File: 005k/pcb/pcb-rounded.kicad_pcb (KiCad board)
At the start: 2 copper layers, 293.2 x 106 mm, 107 parts, among them J1 Screw_Terminal_01x04, U1 ProMicro

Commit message: dim. 10 déc. 2023 13:12:07 CET
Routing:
- net C6: track 234.3 -> 222.5 mm
- net C5: track 287.5 -> 298.1 mm
- net C1: track 426.7 -> 416.5 mm
- net C3: track 419.0 -> 424.1 mm
- net L8: track 210.1 -> 214.1 mm
- net L5: track 143.8 -> 145.8 mm
- net C4: track 334.0 -> 336.0 mm
- net L7: track 153.2 -> 155.0 mm
- net L6: track 138.0 -> 139.7 mm
- net C2: track 438.7 -> 437.7 mm, vias 1 -> 0
- net L1: track 159.0 -> 158.3 mm

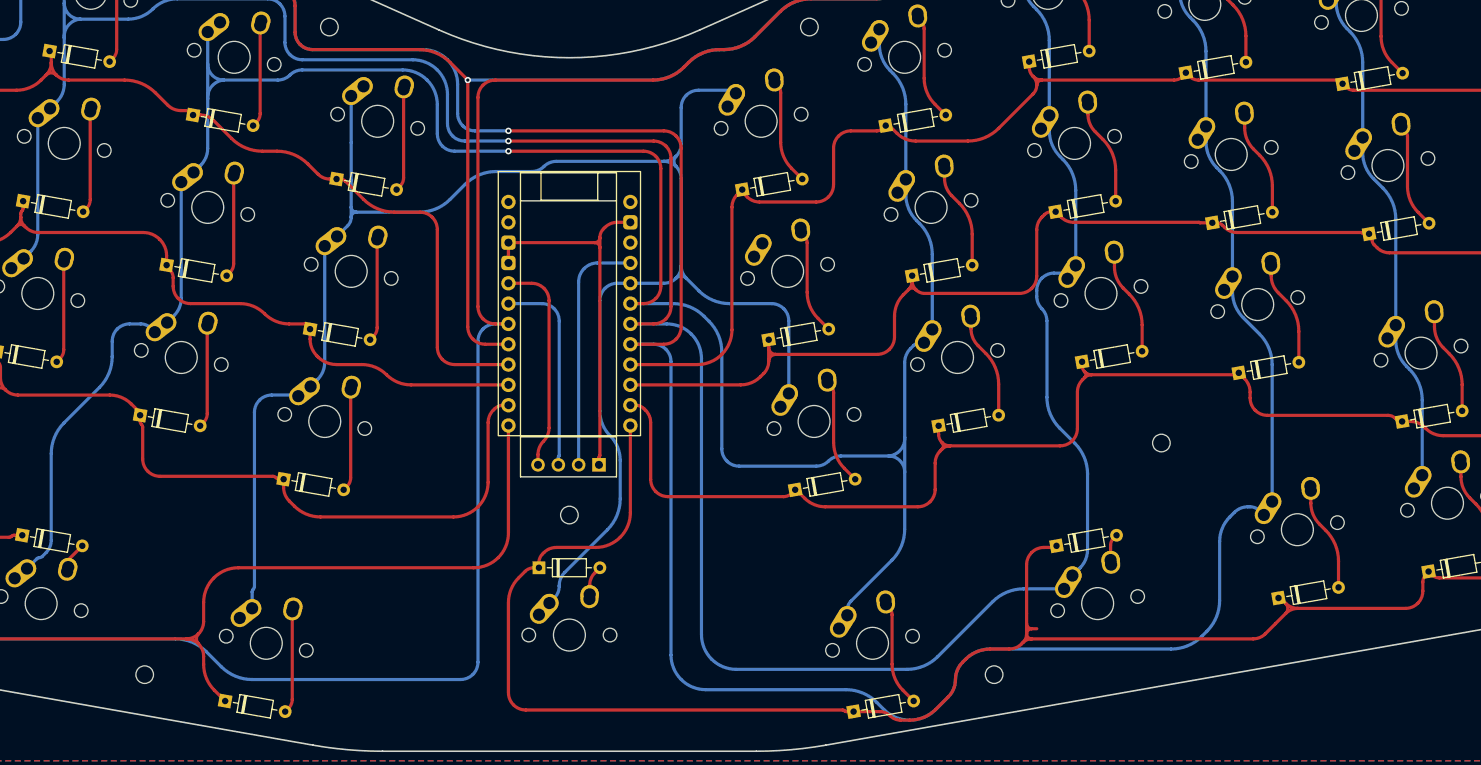
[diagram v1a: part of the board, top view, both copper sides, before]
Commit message: dim. 10 déc. 2023 20:23:19 CET
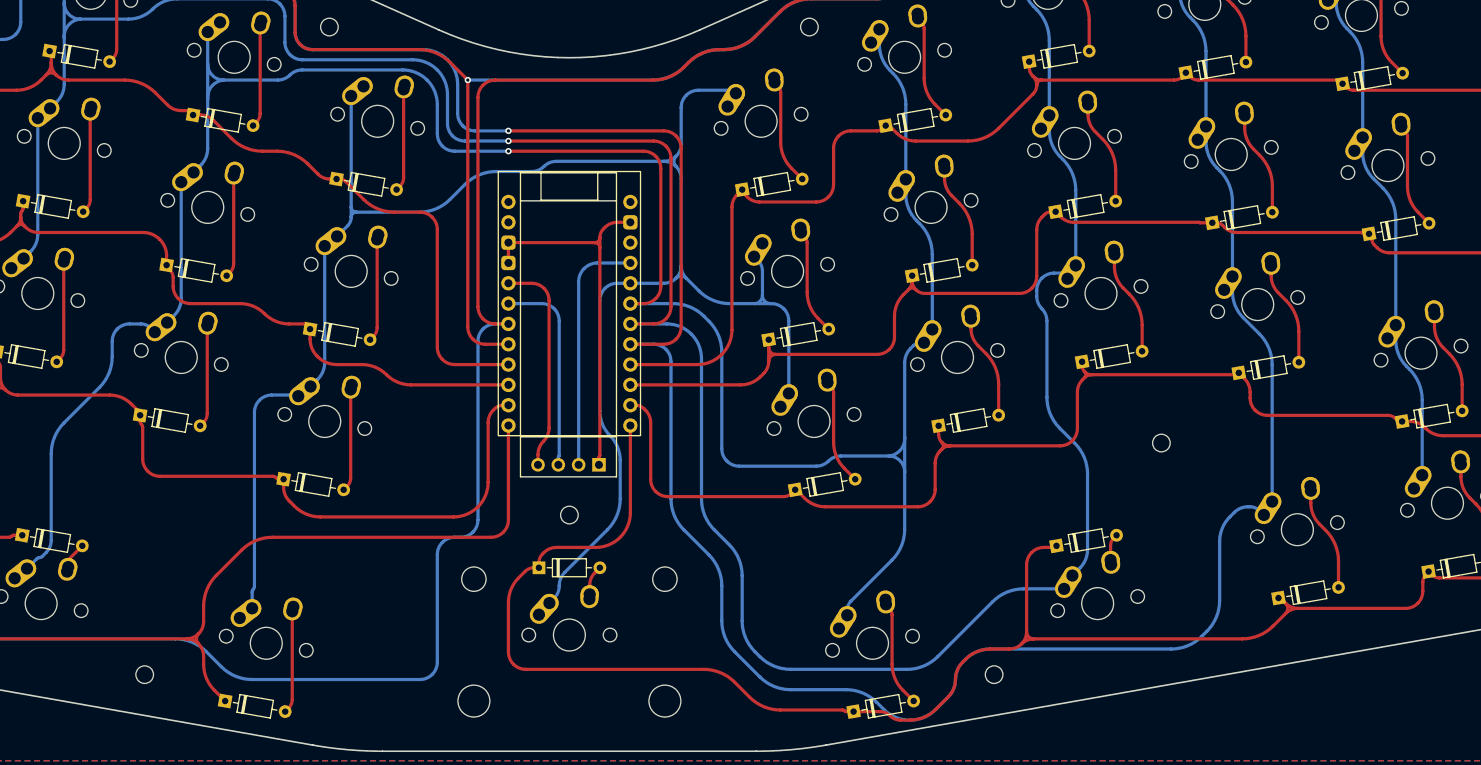
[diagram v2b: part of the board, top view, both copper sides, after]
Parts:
- MX1, MX12, MX13, MX24, MX25, MX36, MX37, MX39, MX40, MX41, MX43, MX44: footprint mx:MX-Alps-Hybrid-1U -> mx:MX-Alps-Hybrid-1.25U
- MX42: footprint mx:MX-Alps-Hybrid-1U -> mx:MX-Alps-Hybrid-2.25U
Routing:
- net C6: track 222.5 -> 230.8 mm
- net C3: track 424.1 -> 417.5 mm
- net L8: track 214.1 -> 208.2 mm
- net C4: track 336.0 -> 331.7 mm
- net C2: track 437.7 -> 435.8 mm
- net L4: track 188.6 -> 187.3 mm
- net L1: track 158.3 -> 157.1 mm
